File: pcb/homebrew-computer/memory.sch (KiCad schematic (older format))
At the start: 15 parts

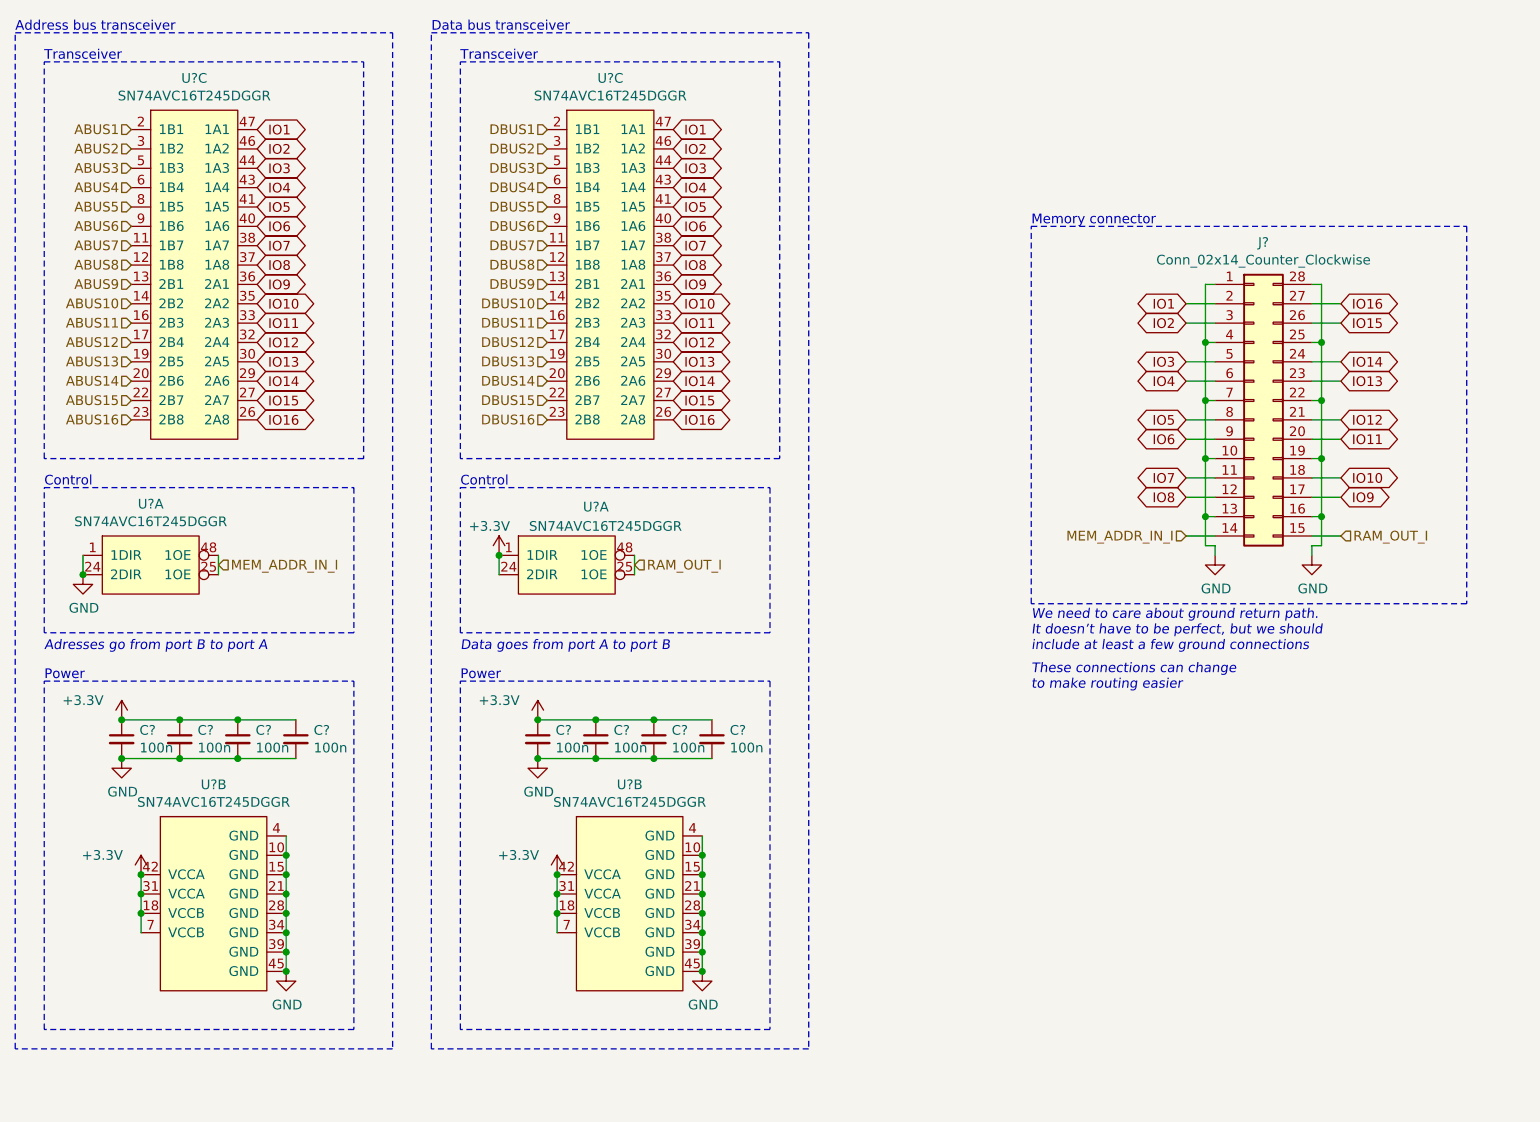
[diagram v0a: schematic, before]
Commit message: Keep working on the peripheral interface
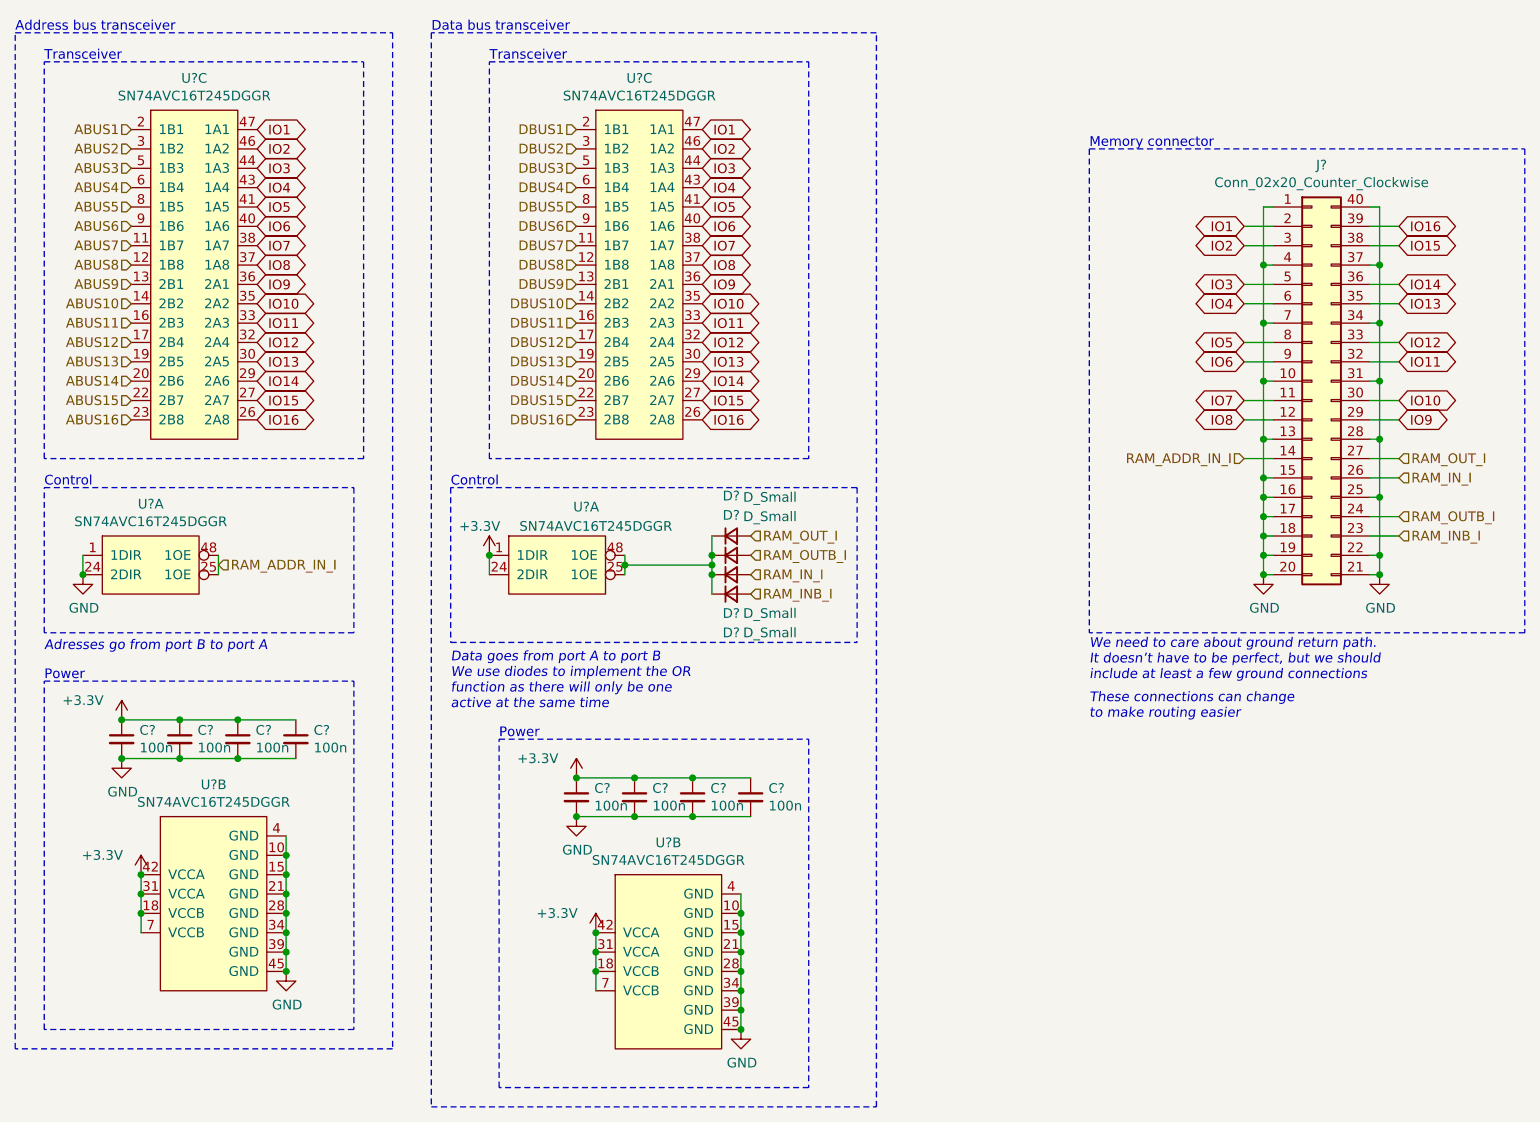
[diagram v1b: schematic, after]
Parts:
- removed J?: Conn_02x14_Counter_Clockwise, symbol Connector_Generic:Conn_02x14_Counter_Clockwise
- added D? (x4): D_Small, symbol Device:D_Small
- added J?: Conn_02x20_Counter_Clockwise, symbol Connector_Generic:Conn_02x20_Counter_Clockwise
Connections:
- net GND: now also J?.1 (Pin_1), J?.10 (Pin_10), J?.13 (Pin_13), J?.15 (Pin_15), J?.16 (Pin_16), J?.17 (Pin_17), J?.18 (Pin_18), J?.19 (Pin_19), J?.20 (Pin_20), J?.21 (Pin_21), J?.22 (Pin_22), J?.25 (Pin_25), J?.28 (Pin_28), J?.31 (Pin_31), J?.34 (Pin_34), J?.37 (Pin_37), J?.4 (Pin_4), J?.40 (Pin_40), J?.7 (Pin_7)
- net IO1: now also J?.2 (Pin_2)
- net IO10: now also J?.30 (Pin_30)
- net IO11: now also J?.32 (Pin_32)
- net IO12: now also J?.33 (Pin_33)
- net IO13: now also J?.35 (Pin_35)
- net IO14: now also J?.36 (Pin_36)
- net IO15: now also J?.38 (Pin_38)
- net IO16: now also J?.39 (Pin_39)
- net IO2: now also J?.3 (Pin_3)
- net IO3: now also J?.5 (Pin_5)
- net IO4: now also J?.6 (Pin_6)
- net IO5: now also J?.8 (Pin_8)
- net IO6: now also J?.9 (Pin_9)
- net IO7: now also J?.11 (Pin_11)
- net IO8: now also J?.12 (Pin_12)
- net IO9: now also J?.29 (Pin_29)
- net RAM_OUT_I: now also D?.2 (A), J?.27 (Pin_27); no longer U?.25 (1OE), U?.48 (1OE)
- net MEM_ADDR_IN_I renamed RAM_ADDR_IN_I
- net RAM_ADDR_IN_I: now also J?.14 (Pin_14)
- new net: D?.1 (K), D?.1 (K), D?.1 (K), D?.1 (K), U?.25 (1OE), U?.48 (1OE)
- new net RAM_INB_I: D?.2 (A), J?.23 (Pin_23)
- new net RAM_IN_I: D?.2 (A), J?.26 (Pin_26)
- new net RAM_OUTB_I: D?.2 (A), J?.24 (Pin_24)
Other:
- note added: "Data goes from port A to port B\nWe use diodes to implement the OR\nfunction as there will only be one \nactive at the same time"
- note removed: "Data goes from port A to port B"
- moved on the sheet: C?, U?A, U?B, U?C
